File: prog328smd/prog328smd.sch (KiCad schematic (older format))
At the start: 5 parts, among them J1 Conn_01x08_Female, J2 Conn_01x08_Female, J3 Conn_01x08_Female, J4 Conn_01x08_Female, U1 ATMEGA328P-AU

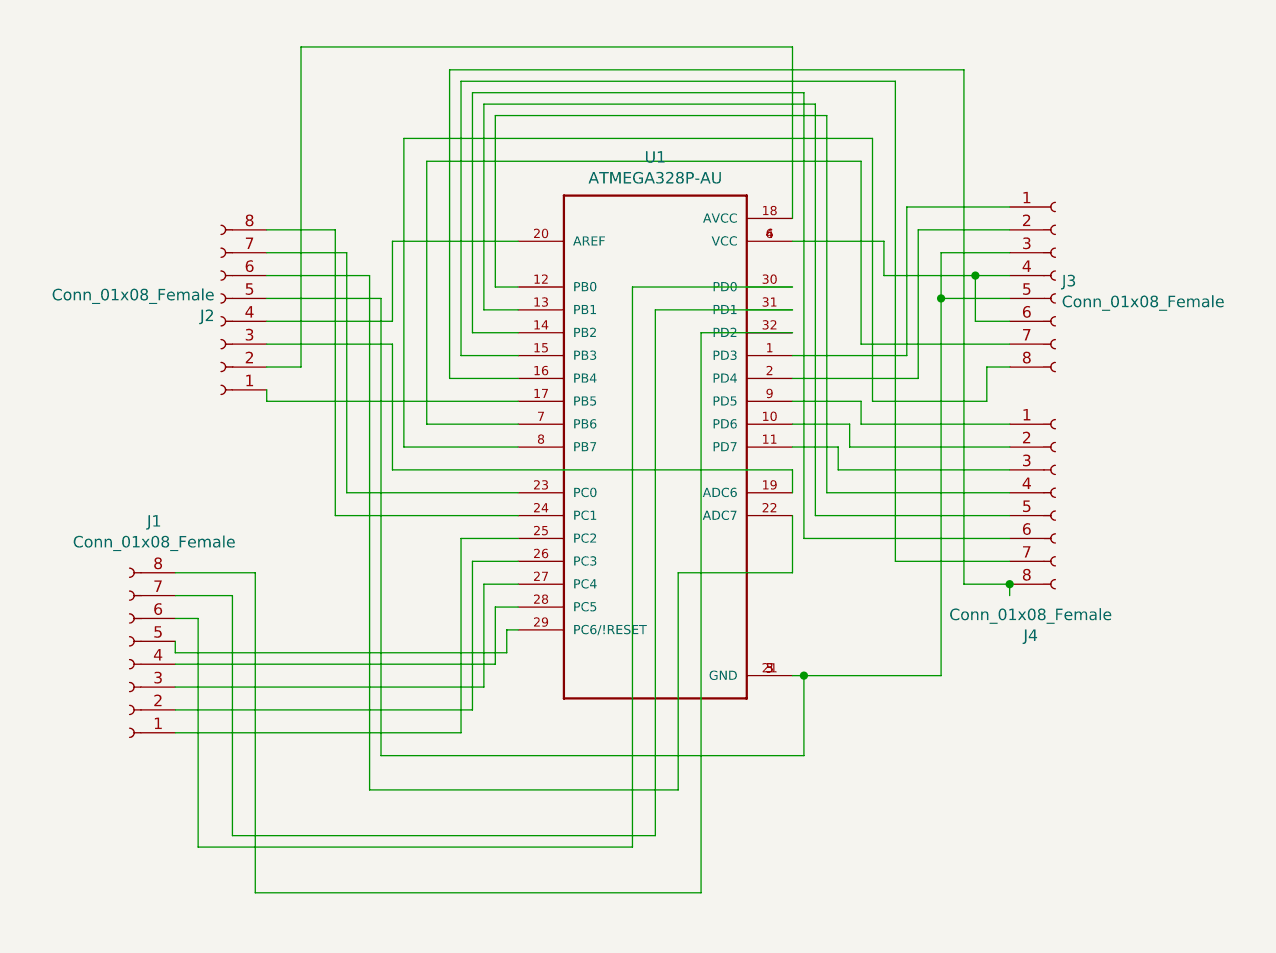
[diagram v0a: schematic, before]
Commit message: First Commit
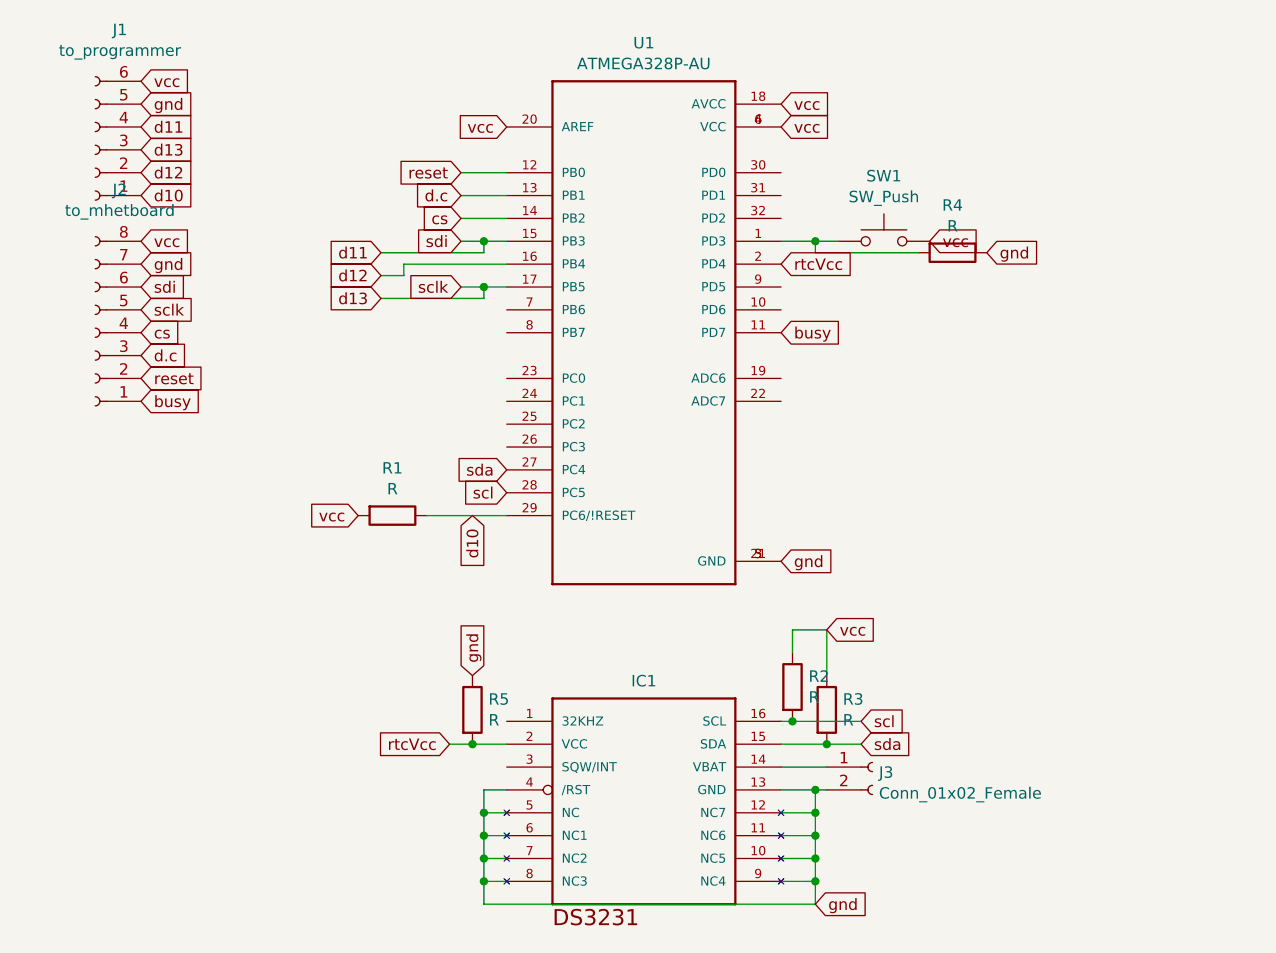
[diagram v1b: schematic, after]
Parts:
- removed J1, J3, J4: Conn_01x08_Female, millk:conn8, symbol Connector:Conn_01x08_Female
- added IC1: DS3231, DS3231:SO16W, symbol DS3231:DS3231
- added J1: to_programmer, millk:conn6, symbol Connector:Conn_01x06_Female
- added J3: Conn_01x02_Female, millk:Conn2, symbol Connector:Conn_01x02_Female
- added R1, R2, R3, R4, R5: R, Resistors_SMD:R_0805_HandSoldering, symbol Device:R
- added SW1: SW_Push, millk:pushbutton_2pin, symbol Switch:SW_Push
- J2: value Conn_01x08_Female -> to_mhetboard
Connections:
- net at U1.1 (PD3): now also R4.2, SW1.1
- net busy: now reaches U1.11 (PD7)
- net busy: now also J2.1 (Pin_1)
- net reset: now reaches U1.12 (PB0)
- net reset: now also J2.2 (Pin_2)
- net d.c: now reaches U1.13 (PB1)
- net d.c: now also J2.3 (Pin_3)
- net cs: now reaches U1.14 (PB2)
- net cs: now also J2.4 (Pin_4)
- net d11: now reaches U1.15 (PB3)
- net d11: now also J2.6 (Pin_6), J1.4 (Pin_4)
- net d12: now reaches U1.16 (PB4)
- net d12: now also J1.2 (Pin_2)
- net d13: now reaches U1.17 (PB5)
- net d13: now also J2.5 (Pin_5), J1.3 (Pin_3); no longer J2.1 (Pin_1)
- net vcc: now reaches U1.18 (AVCC)
- net vcc: now also J2.8 (Pin_8), U1.20 (AREF), U1.4 (VCC), U1.6 (VCC), J1.6 (Pin_6), R1.2, R2.1, R3.1, SW1.2; no longer J2.2 (Pin_2)
- net at U1.19 (ADC6): no longer J2.3 (Pin_3)
- net rtcVcc: now reaches U1.2 (PD4)
- net rtcVcc: now also IC1.2 (VCC), R5.2
- net gnd: now reaches U1.21 (GND), U1.3 (GND), U1.5 (GND)
- net gnd: now also J2.7 (Pin_7), IC1.10 (NC5), IC1.11 (NC6), IC1.12 (NC7), IC1.13 (GND), IC1.4 (/RST), IC1.5 (NC), IC1.6 (NC1), IC1.7 (NC2), IC1.8 (NC3), IC1.9 (NC4), J1.5 (Pin_5), J3.2 (Pin_2), R4.1, R5.1; no longer J2.5 (Pin_5)
- net at U1.22 (ADC7): no longer J2.6 (Pin_6)
- net at U1.23 (PC0): no longer J2.7 (Pin_7)
- net at U1.24 (PC1): no longer J2.8 (Pin_8)
- net sda: now reaches U1.27 (PC4)
- net sda: now also IC1.15 (SDA), R3.2
- net scl: now reaches U1.28 (PC5)
- net scl: now also IC1.16 (SCL), R2.2
- net d10: now reaches U1.29 (PC6/!RESET)
- net d10: now also J1.1 (Pin_1), R1.1
- new net: IC1.14 (VBAT), J3.1 (Pin_1)
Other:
- moved on the sheet: U1
